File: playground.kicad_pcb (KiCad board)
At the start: 2 copper layers, 80 x 50 mm, 39 parts, among them IC1 TXU0101DBVR, IC10 TPS562242DRLR, IC2 TXU0101DBVR, IC3 TXU0101DBVR, IC4 TXU0101DBVR, IC5 TXU0101DBVR, IC6 TXU0101DBVR, IC7 TXU0101DBVR, IC8 TXU0101DBVR, IC9 L293DD, J2 Pump, J3 Fan, J4 Valve, J6 MOLEX POWER CONNECTOR, J7 USB_A, SW1 SW_DIP_x01, U2 ATSAMD21G18A-A

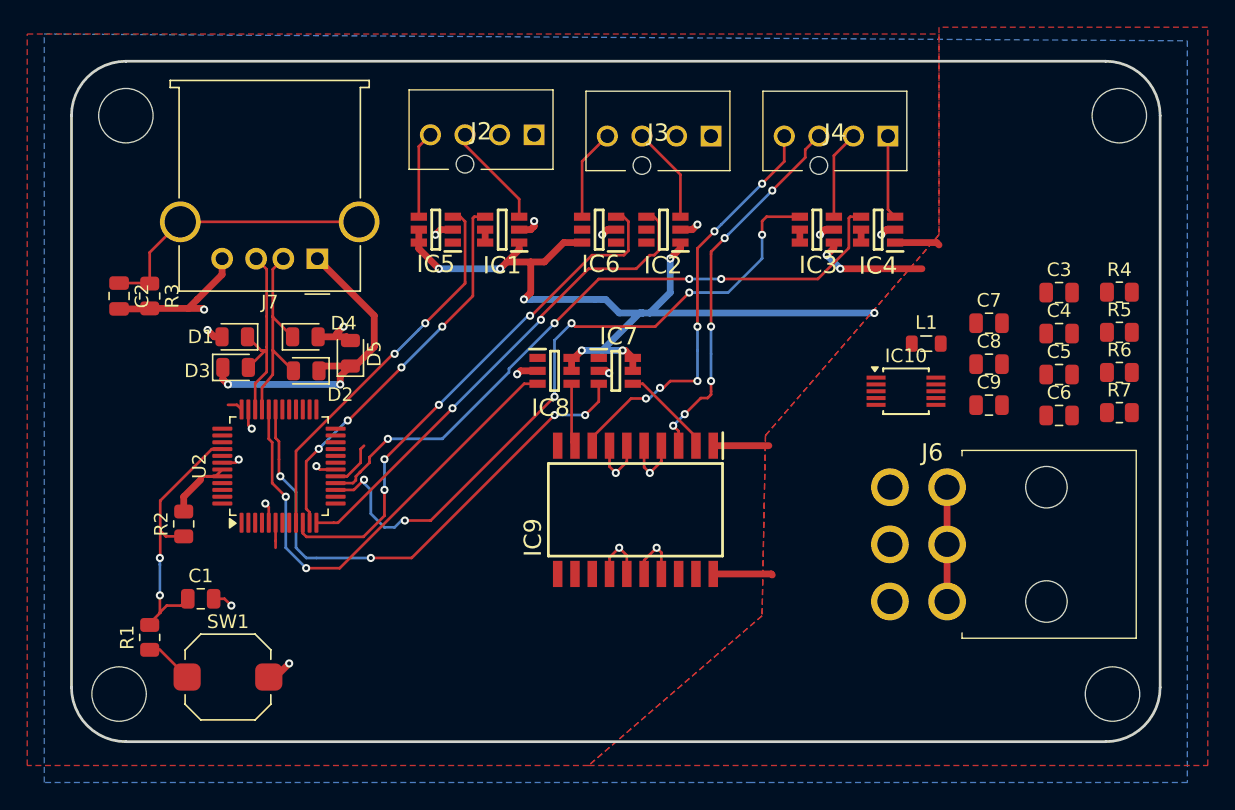
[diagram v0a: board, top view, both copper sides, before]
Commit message: saving progress
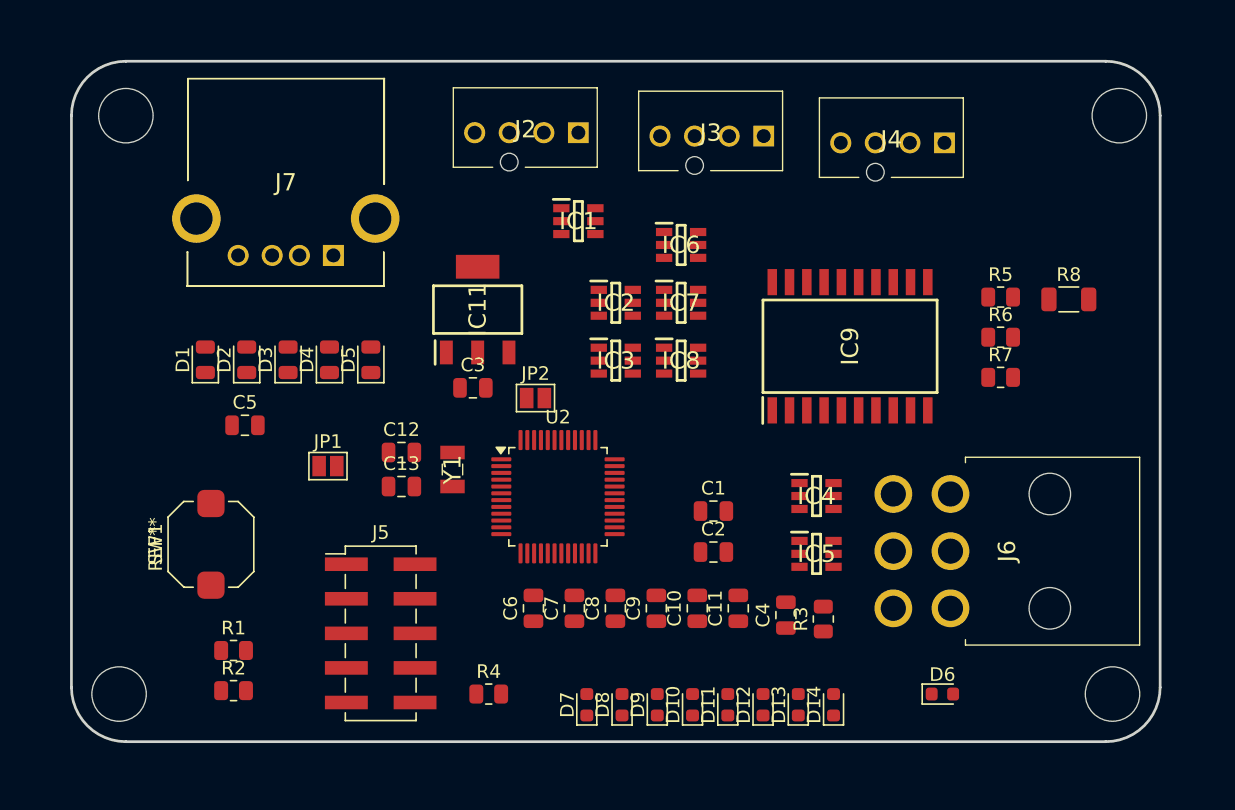
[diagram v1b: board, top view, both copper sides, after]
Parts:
- removed IC10: TPS562242DRLR, Package_SO:MSOP-10_3x3mm_P0.5mm
- removed L1: 3u3, Inductor_SMD:L_0805_2012Metric
- added C10: 10u, Capacitor_SMD:C_0805_2012Metric, F.Cu at (146.0, 90.2)
- added C11: 10u, Capacitor_SMD:C_0805_2012Metric, F.Cu at (149.0, 90.2)
- added C12: 20p, Capacitor_SMD:C_0805_2012Metric, F.Cu at (124.2, 78.8)
- added C13: 20p, Capacitor_SMD:C_0805_2012Metric, F.Cu at (124.2, 81.2)
- added D10: FAN_PWM_IND, LED_SMD:LED_0603_1608Metric, F.Cu at (145.6, 97.3)
- added D11: VALVE_OPEN_IND, LED_SMD:LED_0603_1608Metric, F.Cu at (148.2, 97.3)
- added D12: VALVE_CLOSED_IND, LED_SMD:LED_0603_1608Metric, F.Cu at (150.8, 97.3)
- added D13: GENERAL_BOARD_1_IND, LED_SMD:LED_0603_1608Metric, F.Cu at (153.4, 97.3)
- added D14: GENERAL_BOARD_1_IND, LED_SMD:LED_0603_1608Metric, F.Cu at (156.0, 97.3)
- added D6: 5V_USB_PWR_IND, LED_SMD:LED_0603_1608Metric, F.Cu at (164.0, 96.5)
- added D7: 3v3_PWR_IND, LED_SMD:LED_0603_1608Metric, F.Cu at (137.9, 97.3)
- added D8: 12v_PWR_IND, LED_SMD:LED_0603_1608Metric, F.Cu at (140.5, 97.3)
- added D9: PUMP_PWM_IND, LED_SMD:LED_0603_1608Metric, F.Cu at (143.1, 97.3)
- added IC11: LM3940IMP-3.3_NOPB, custom_footprints:SOT230P700X180-4N, F.Cu at (129.8, 68.2)
- added J5: Conn_02x05_Counter_Clockwise, Connector_PinHeader_2.54mm:PinHeader_2x05_P2.54mm_Vertical_SMD, F.Cu at (122.7, 92.0)
- added JP1: SolderJumper_2_Open, Jumper:SolderJumper-2_P1.3mm_Open_Pad1.0x1.5mm, F.Cu at (118.8, 79.8)
- added JP2: SolderJumper_2_Open, Jumper:SolderJumper-2_P1.3mm_Open_Pad1.0x1.5mm, F.Cu at (134.1, 74.8)
- added R8: 300R, Resistor_SMD:R_1206_3216Metric, F.Cu at (173.3, 67.5)
- added Y1: 32.768kHz, custom_footprints:FC135327680KAA5, F.Cu at (128.0, 80.0)
- C1: value C -> 100n
- C3: value 10u -> 4.7n
- C4: value 10u -> 100n
- C5: value 100n -> 47u
- C7: value 33p -> 100n
- C8: value 22u -> 1u
- C9: value 100n -> 1u
- J7: footprint Connector_USB:USB_A_Molex_67643_Horizontal -> custom_footprints:676432910
- R4: value 100k -> 1k
- R5: value 11k3 -> 51R
- R6: value 158k -> 470R
- R7: value 30k -> 470R
- moved C5 59.9 mm to (112.8, 76.8)
- moved R4 55.0 mm to (130.7, 96.5)
- moved R3 54.9 mm to (155.2, 91.0), turned to 90 degrees
- moved C2 47.6 mm to (147.2, 86.1), turned to 0 degrees
- moved C3 43.6 mm to (129.5, 74.0)
- moved C6 41.1 mm to (133.9, 90.2), turned to 90 degrees
- moved C1 38.2 mm to (147.2, 83.1)
- moved C7 37.0 mm to (137.0, 90.2), turned to 90 degrees
- moved IC5 36.7 mm to (154.8, 86.2), turned to 0 degrees
- moved C8 32.8 mm to (140.0, 90.2), turned to 90 degrees
- moved C4 28.8 mm to (152.5, 90.7), turned to 90 degrees
- moved C9 28.6 mm to (143.0, 90.2), turned to 90 degrees
- moved U2 20.6 mm to (135.8, 82.0), turned to 0 degrees
- moved IC4 20.1 mm to (154.8, 82.0), turned to 0 degrees
- moved IC9 19.8 mm to (157.2, 70.9), turned to 90 degrees
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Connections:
- C3 pad 1: +12V -> /LDO_POWER_IN
- C4 pad 1: +12V -> +3V3
- C5 pad 1: +12V -> /LDO_POWER_OUT
- C6 pad 1: /Power Regulation/buck_sw -> +3V3
- C6 pad 2: Net-(IC10-BST) -> GND
- C7 pad 1: /Power Regulation/buck_fb -> +3V3
- C7 pad 2: +5V -> GND
- C8 pad 1: GND -> +3V3
- C8 pad 2: +5V -> GND
- C9 pad 1: GND -> +3V3
- C9 pad 2: +5V -> GND
- D1 pad 1: /USB_VBUS -> +5V
- D2 pad 1: /USB_VBUS -> +5V
- D5 pad 1: /USB_VBUS -> +5V
- J7 pad 1: /USB_VBUS -> +5V
- R4 pad 1: +12V -> /SWCLK
- R4 pad 2: /Power Regulation/buck_en -> +3V3
- R5 pad 1: /Power Regulation/buck_en -> GND
- R5 pad 2: GND -> +3V3
- R6 pad 1: +5V -> Net-(R6-Pad1)
- R6 pad 2: /Power Regulation/buck_fb -> +12V
- R7 pad 1: /Power Regulation/buck_fb -> Net-(R6-Pad1)
- U2 pad 1: unconnected-(U2-PA00-Pad1) -> /XIN32
- U2 pad 2: unconnected-(U2-PA01-Pad2) -> /XOUT32
- U2 pad 45: unconnected-(U2-PA30-Pad45) -> /SWCLK
- U2 pad 46: unconnected-(U2-PA31-Pad46) -> /SWDIO
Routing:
- net +5V: track 83.1 -> 0.00 mm, vias 9 -> 0
- net GND: track 54.2 -> 0.00 mm, vias 21 -> 0
- net /ValveSense1_3v3: track 50.7 -> 0.00 mm, vias 6 -> 0
- net /ValveSense2_3v3: track 48.8 -> 0.00 mm, vias 4 -> 0
- net /ValveCtrl1_3v3: track 39.4 -> 0.00 mm, vias 4 -> 0
- net /FanCtrl_3v3: track 39.1 -> 0.00 mm, vias 4 -> 0
- net /FanSense_3v3: track 36.8 -> 0.00 mm, vias 2 -> 0
- net /ValveCtrl2_3v3: track 35.4 -> 0.00 mm, vias 2 -> 0
- net /ValveOutput2_12v: track 30.7 -> 0.00 mm, vias 6 -> 0
- net /PumpSense_3v3: track 28.6 -> 0.00 mm, vias 4 -> 0
- net /PumpCtrl_3v3: track 28.4 -> 0.00 mm, vias 2 -> 0
- net /ValveOutput1_12v: track 27.6 -> 0.00 mm, vias 6 -> 0
- net /USB_VBUS: track 24.3 -> 0.00 mm, vias 2 -> 0
- net /usb_shield_gnd: track 20.9 -> 0.00 mm
- net /RESET: track 20.0 -> 0.00 mm, vias 2 -> 0
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- removed copper zone on F.Cu, net +3V3
- removed copper zone on F.Cu, net +5V
- removed copper zone on B.Cu, net GND
